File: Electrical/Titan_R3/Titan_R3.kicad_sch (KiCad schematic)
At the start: 99 parts, among them IC1 NEO-M9N-00B, J1 BATT, J10 UART, J11 SPI, J12 PROPY, J13 PROPZ, J14 TVCY, J15 GPS ANT, J16 TVCZ, J17 PYRO 1, J18 PYRO 2, J19 PYRO 3, J2 12V OUT, J20 PYRO 4, J21 DM3D-SF, J3 USB_C_Receptacle_USB2.0, J4 5V OUT, J5 SW, J6 3V3 OUT, J7 PYRO ARM, J8 SWD, J9 I2C, Q1 PYRO 1, Q2 PYRO 2, Q3 PYRO 3, Q4 PYRO 4, U1 AP63300WU-7, U2 AZ1117-3.3, U3 USBLC6-2P6, U4 ATSAMD51J19A-A, U5 BMP280, U6 SST26VF032B-104I_SM, U7 BMI088, U8 LSM9DS1TR, Y1 32.768

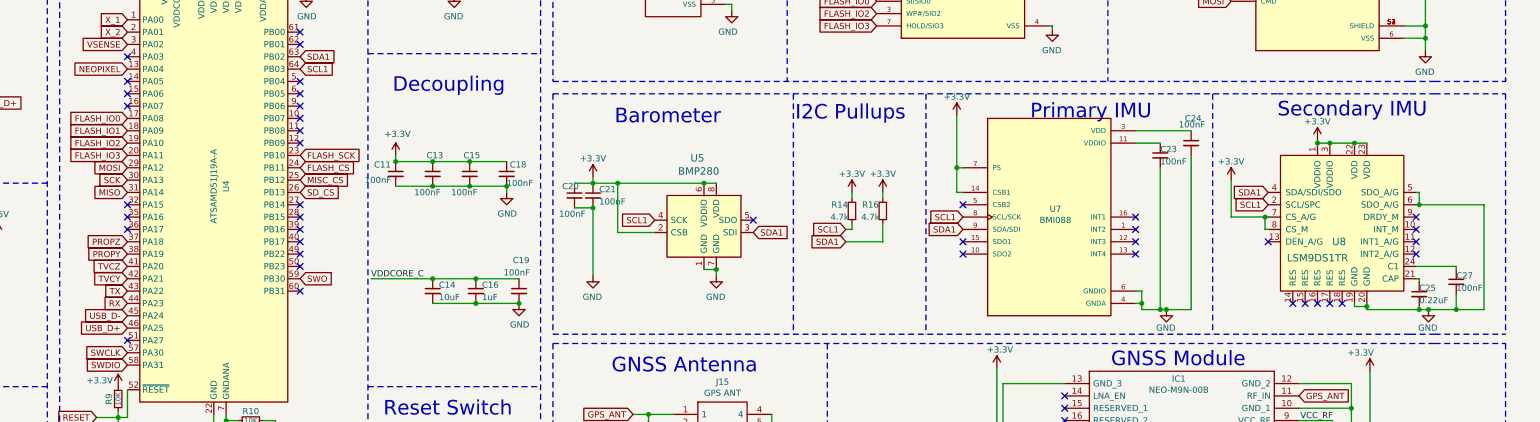
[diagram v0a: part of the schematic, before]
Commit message: major flight software changes
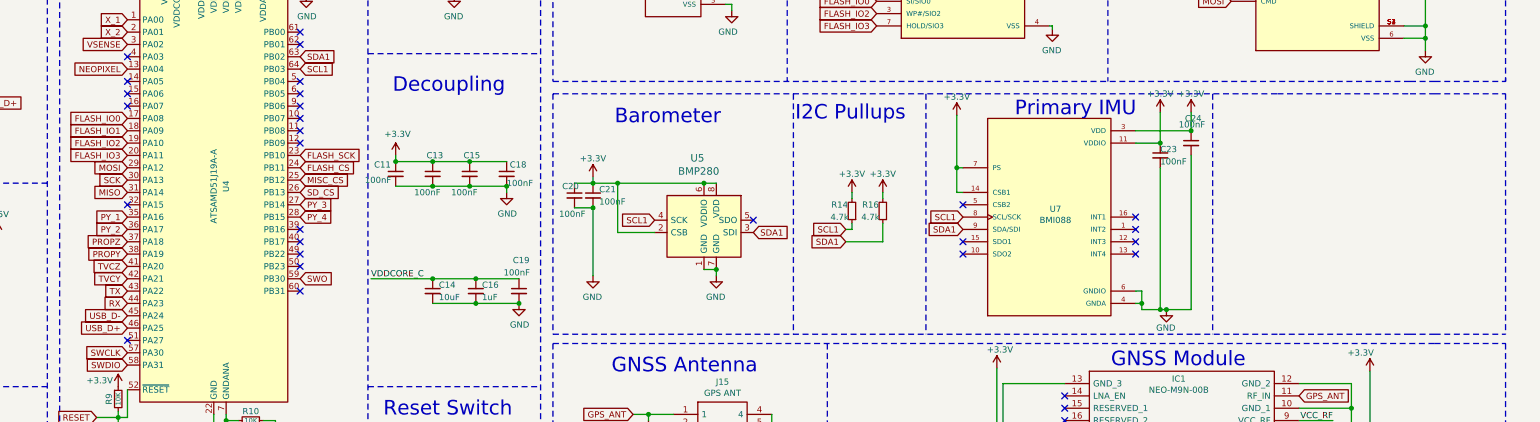
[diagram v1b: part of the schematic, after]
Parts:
- removed C25: 0.22uF, Capacitor_SMD:C_0603_1608Metric, symbol Device:C_Small
- removed C27: 100nF, Capacitor_SMD:C_0603_1608Metric, symbol Device:C_Small
- removed U8: LSM9DS1TR, digikey-footprints:LGA-24_3x3.5mm_LSM9DS1, symbol dk_Motion-Sensors-IMUs-Inertial-Measurement-Units:LSM9DS1TR
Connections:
- net +3V3: now also C23.1, C24.1, U7.11 (VDDIO), U7.3 (VDD)
- net PY_1: now also U4.35 (PA16)
- net PY_2: now also U4.36 (PA17)
- net PY_3: now also U4.27 (PB14)
- net PY_4: now also U4.28 (PB15)
- no-connect marks 72 -> 58
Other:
- note removed: "Secondary IMU"
